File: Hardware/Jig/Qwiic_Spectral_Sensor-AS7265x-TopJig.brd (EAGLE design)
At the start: 35.6 x 40.6 mm, 93 parts, among them J2 Serial Interface, J5 Flash Programming, J8 PTH, U1 AS72651, U3 4MB Flash, U5 AS72653, U6 AS72652

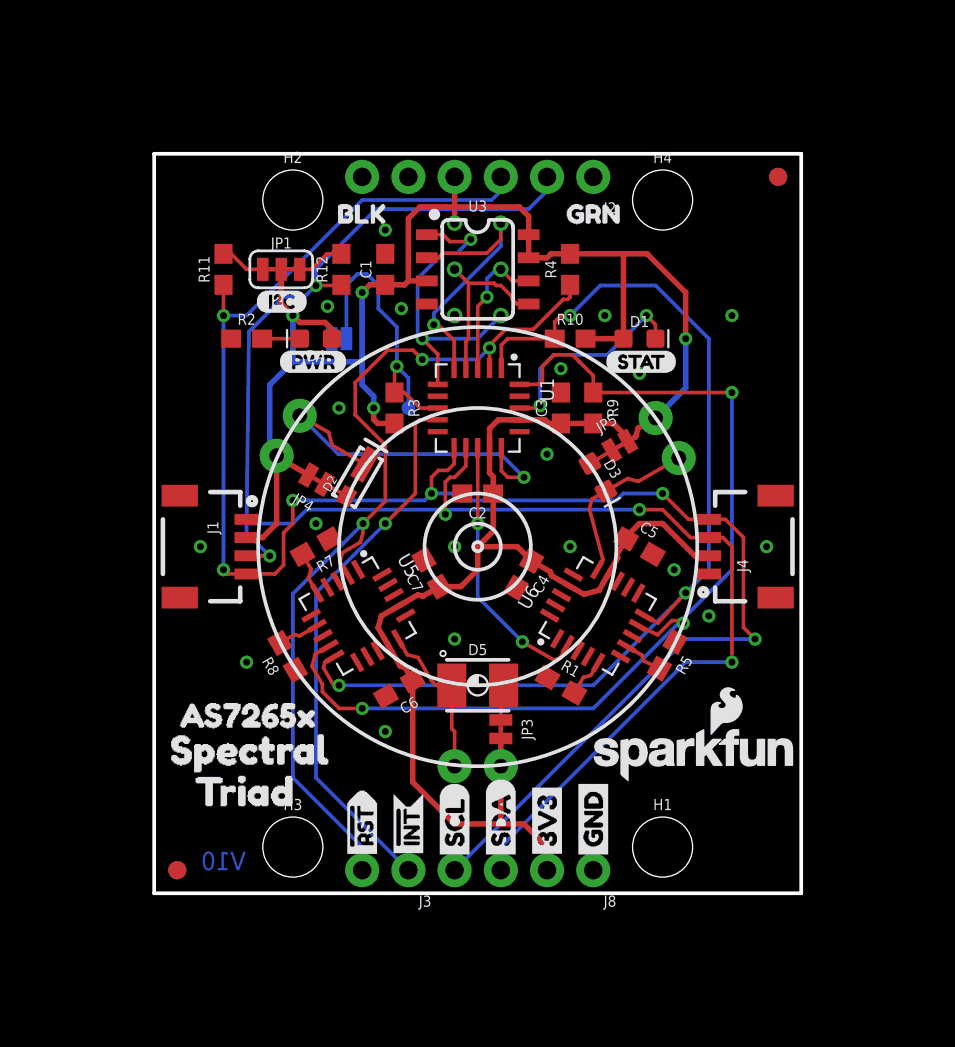
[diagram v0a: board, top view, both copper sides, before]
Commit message: Silk changes before panelization
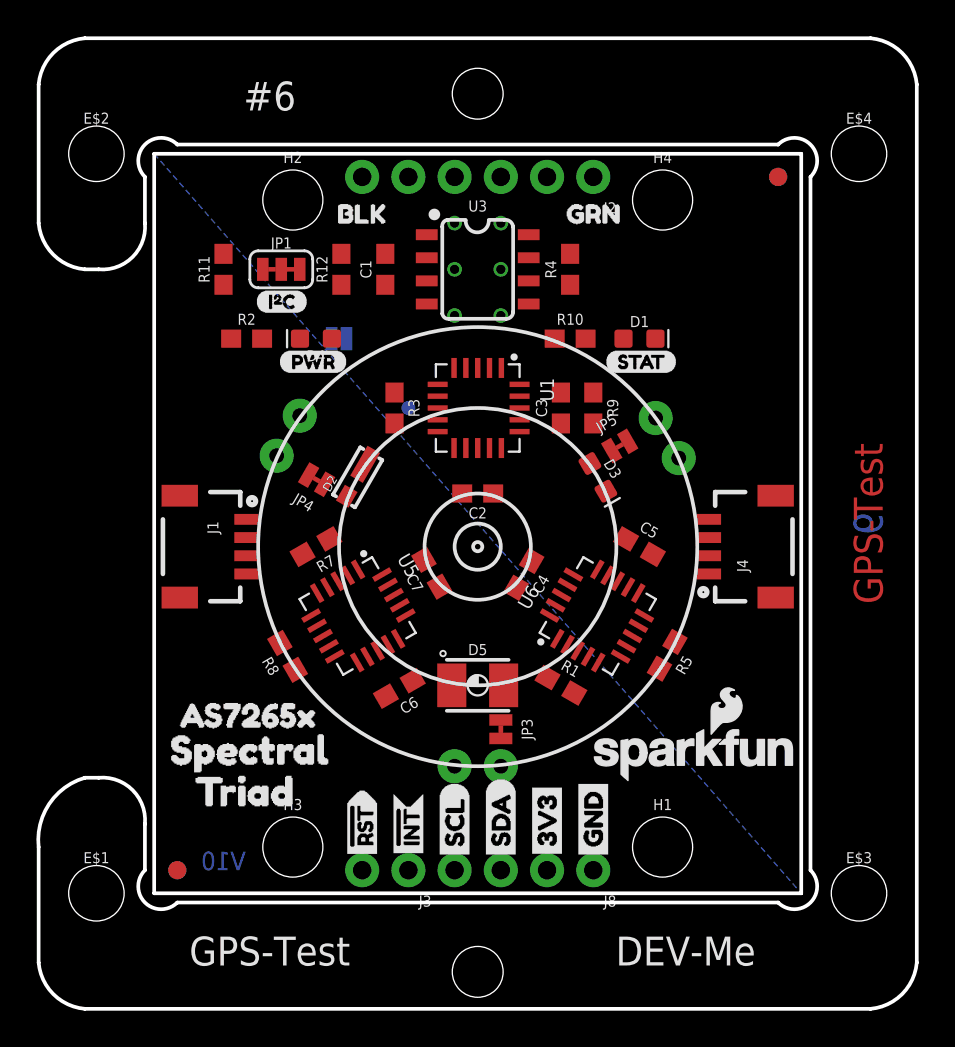
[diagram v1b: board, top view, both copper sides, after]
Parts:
- removed U$1, U$36, U$37: (no value), buzzard_labels (7):#0
- removed U$38, U$39, U$40: (no value), buzzard_labels (7):#1
- added E$1, E$2, E$3, E$4: (no value), SparkFun-Hardware:STAND-OFF-TIGHT
- added E$5, E$6: (no value), SparkFun-Hardware:NUBBIN_LOCKER
- D2: device SparkFun-LED:SUPER_BRIGHT_SMD_LED_3014 -> SparkX:SUPER_BRIGHT_SMD_LED_1206
- moved U$6 0.25 mm to (28.1, 21.3)
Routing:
- net 3.3V: track 143.3 -> 0.00 mm, vias 4 -> 0
- net RX/SCL: track 99.0 -> 0.00 mm, vias 6 -> 0
- net TX/SDA: track 93.2 -> 0.00 mm, vias 5 -> 0
- net SDA_S: track 56.9 -> 0.00 mm, vias 3 -> 0
- net SCL_S: track 56.2 -> 0.00 mm, vias 3 -> 0
- net !RST: track 50.8 -> 0.00 mm, vias 3 -> 0
- net !INT: track 30.2 -> 0.00 mm, vias 1 -> 0
- net LED_DRV: track 21.0 -> 0.00 mm, vias 1 -> 0
- net !CS_EE: track 17.6 -> 0.00 mm, vias 2 -> 0
- net I2C_ENB: track 16.8 -> 0.00 mm, vias 1 -> 0
- net MISO: track 15.5 -> 0.00 mm, vias 1 -> 0
- net !RST-ADDR: track 14.9 -> 0.00 mm, vias 2 -> 0
- net N$2: track 11.8 -> 0.00 mm, vias 2 -> 0
- net MOSI: track 9.65 -> 0.00 mm
- net LED_DRV1: track 9.51 -> 0.00 mm
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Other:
- board size 35.6 x 40.6 mm -> 48.3 x 53.3 mm
- board text added: "#6"
- board text added: "6"
- board text added: "DEV-Me"
- board text added: "GPS-Test"
